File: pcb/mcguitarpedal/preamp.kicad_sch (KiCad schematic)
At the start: 25 parts, among them J8 POT_HP_VOLUME_10k, U3 LM4562

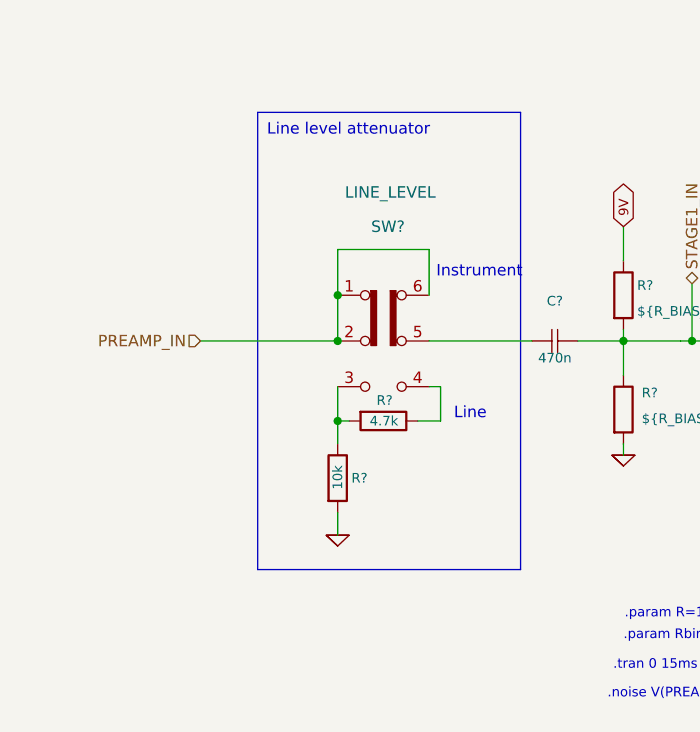
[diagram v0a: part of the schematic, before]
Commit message: Miniaturization
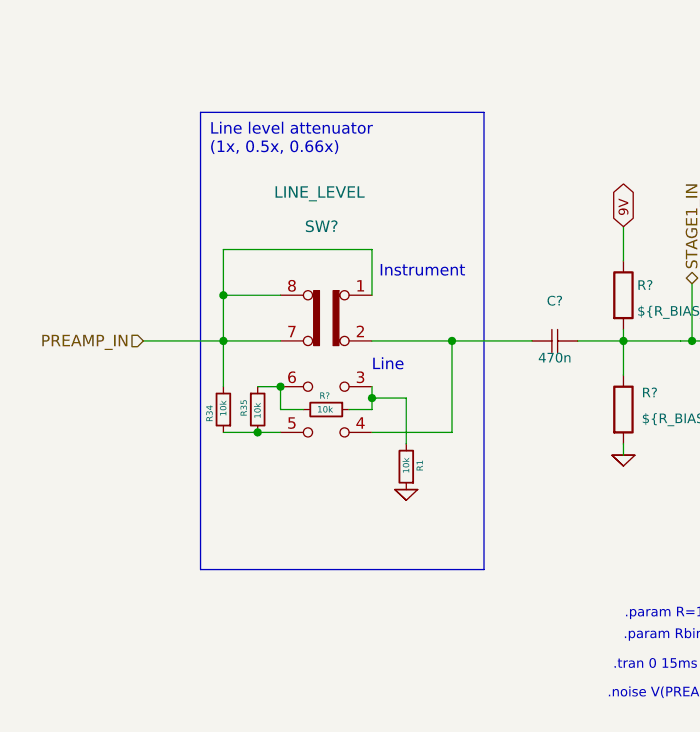
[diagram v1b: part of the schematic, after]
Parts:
- removed R?: 10k, Resistor_THT:R_Axial_DIN0207_L6.3mm_D2.5mm_P7.62mm_Horizontal, symbol Device:R
- added R1, R34, R35: 10k, Resistor_SMD:R_1206_3216Metric_Pad1.30x1.75mm_HandSolder, symbol Device:R_Small
- R?: value 4.7k -> 10k; footprint Resistor_THT:R_Axial_DIN0207_L6.3mm_D2.5mm_P7.62mm_Horizontal -> Resistor_SMD:R_1206_3216Metric_Pad1.30x1.75mm_HandSolder; symbol Device:R -> Device:R_Small
- SW?: footprint Button_Switch_THT:SW_CK_JS202011AQN_DPDT_Angled -> mcguitarpedal:DP3T slide switch; symbol Switch:SW_Slide_DPDT -> mcguitarpedal:SW_Slide_DP3T
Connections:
- net 0: now also R1.1
- net PREAMP_IN: now also SW?.7 (B), SW?.8 (C), R34.2; no longer SW?.2 (B), SW?.6 (C)
- net at SW?.3 (C): now also R?.1, R1.2; no longer R?.2
- net at SW?.4 (D): now also C?.2, SW?.2 (B); no longer R?.1
- net at SW?.5: now also R34.1, R35.2; no longer C?.2
- new net: R35.1, R?.2, SW?.6 (A)
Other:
- moved on the sheet: R?
